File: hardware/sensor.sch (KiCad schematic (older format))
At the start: 43 parts, among them P1 CONN_01X05, SW1 Reset, U2 CD74HC4046, U3 CD74HC4046, U4 Atmel_SAM_D09, X1 UART

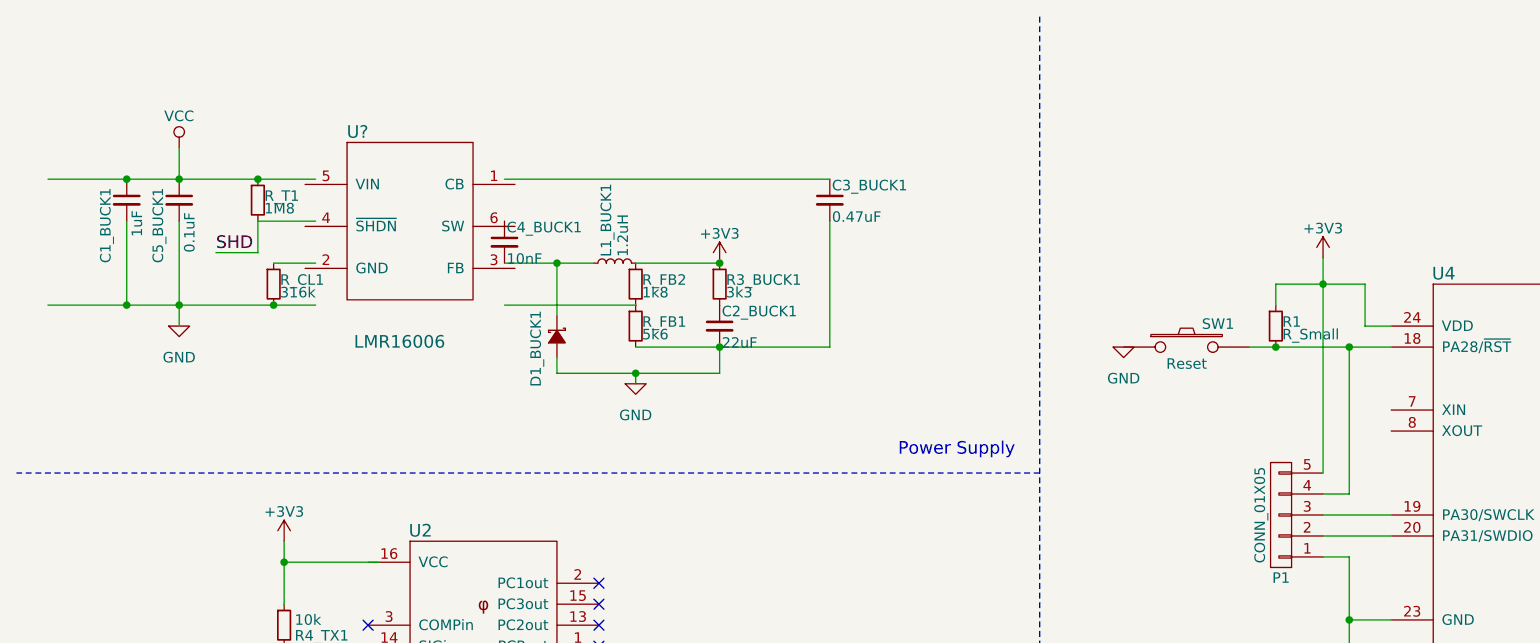
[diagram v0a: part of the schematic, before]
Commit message: New buck schema is done
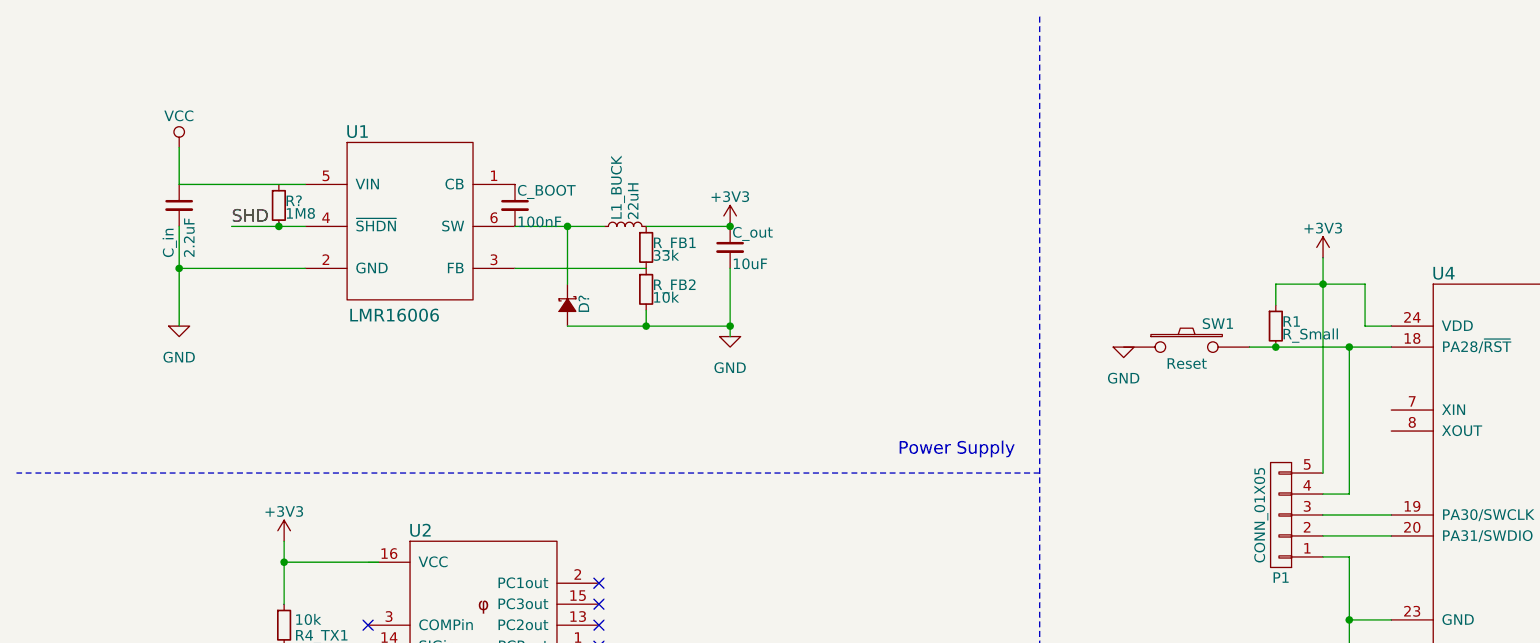
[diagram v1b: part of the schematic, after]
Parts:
- removed C1_BUCK1: 1uF, Capacitors_SMD:C_0805, symbol C_Small
- removed C3_BUCK1: 0.47uF, Capacitors_SMD:C_0603, symbol C_Small
- removed D1_BUCK1: D_Schottky_Small, symbol D_Schottky_Small
- removed R3_BUCK1: 3k3, symbol R_Small
- removed R_CL1: 316k, symbol R_Small
- added D?: D_Schottky_Small, symbol D_Schottky_Small
- C_BOOT: renamed from C4_BUCK1; value 10nF -> 100nF
- C_in: renamed from C5_BUCK1; value 0.1uF -> 2.2uF
- C_out: renamed from C2_BUCK1; value 22uF -> 10uF
- L1_BUCK: renamed from L1_BUCK1; value 1.2uH -> 22uH
- R_FB1: renamed from R_FB2; value 1k8 -> 33k
- R_FB2: renamed from R_FB1; value 5k6 -> 10k
- gave numbers to parts that had none: 1
- renumbered R_T1 to R?
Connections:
- wire segments 81 -> 73
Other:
- moved on the sheet: C_BOOT, C_in, C_out, L1_BUCK, R?, R_FB1, R_FB2
